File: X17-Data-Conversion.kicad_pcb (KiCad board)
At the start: 2 copper layers, 41.5 x 30.7 mm, 28 parts, among them J1 Conn_01x05, J4 Conn_01x12_Pin, U2 STM32F091CCTx, U3 MAX485E, U4 MAX7375AXR805+T, U5 AZ1117IH-3.3TRG1

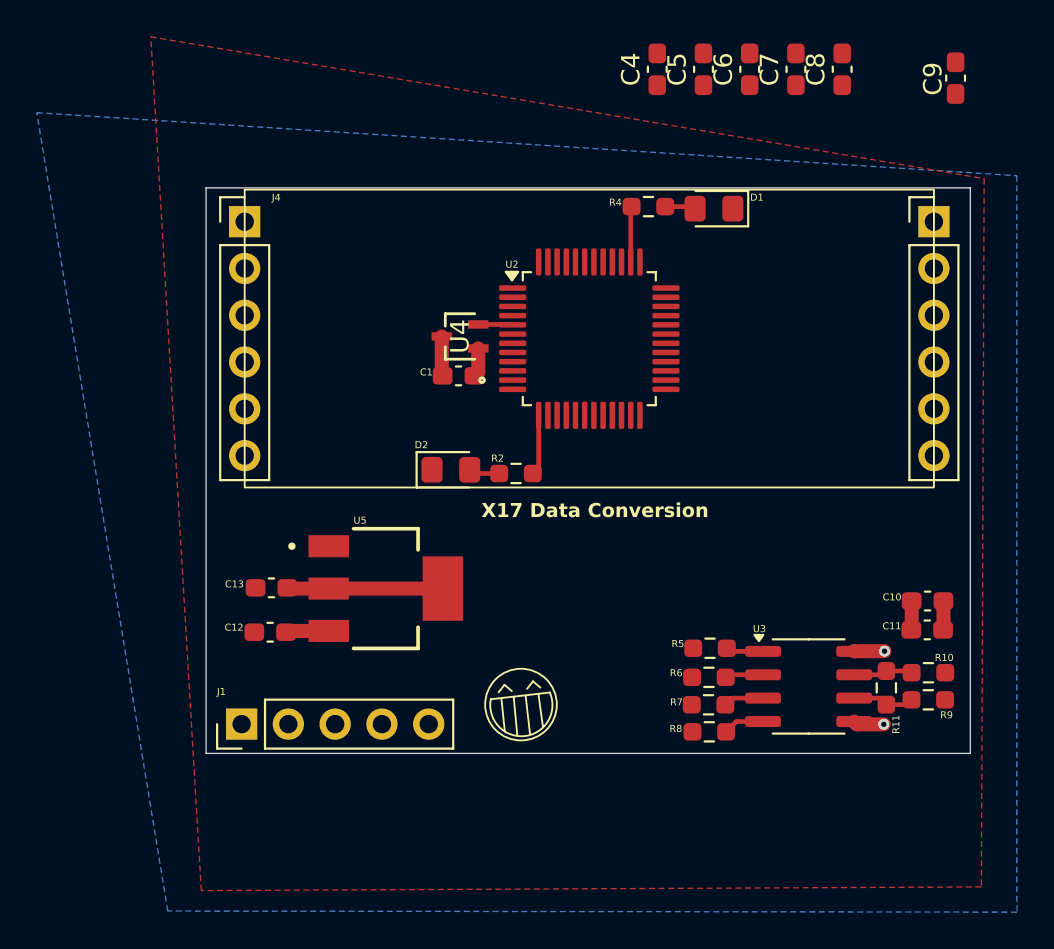
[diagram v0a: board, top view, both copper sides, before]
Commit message: goodie
going good
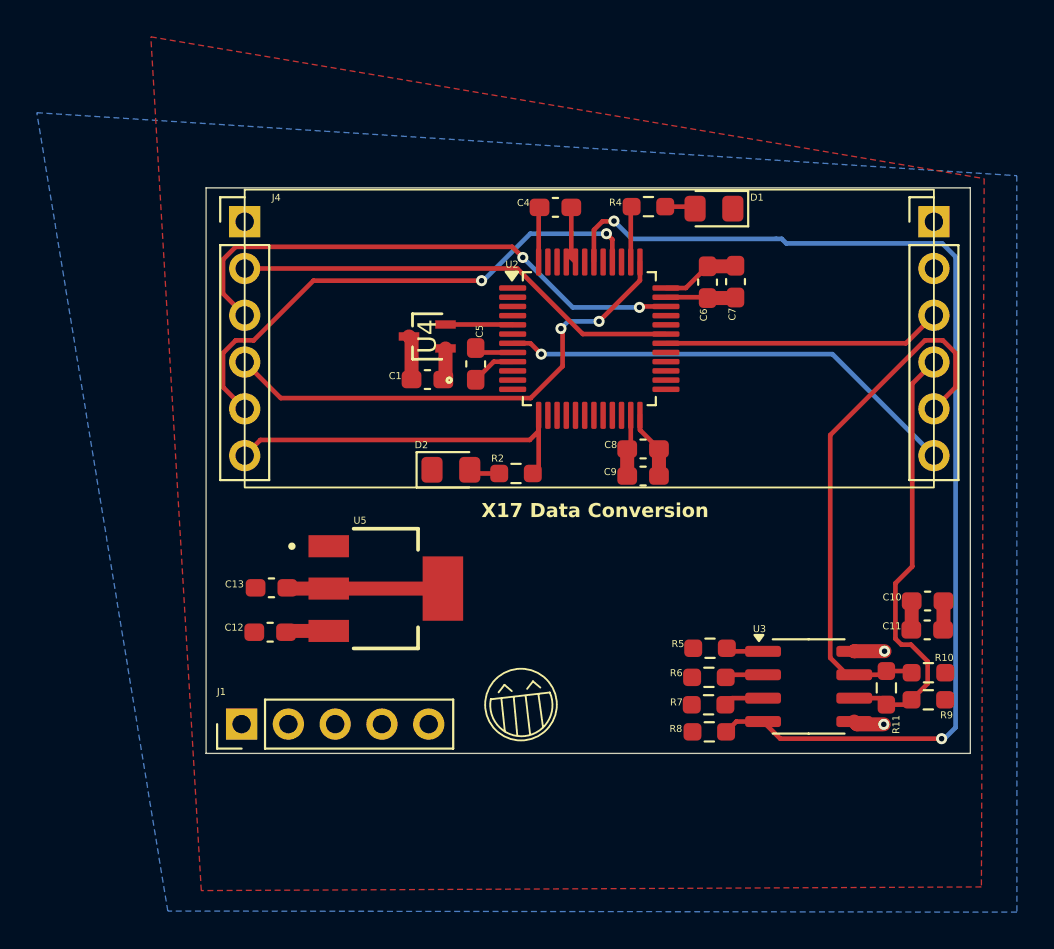
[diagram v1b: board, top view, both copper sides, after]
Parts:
- moved C9 27.5 mm to (164.5, 81.7), turned to 0 degrees
- moved C8 23.3 mm to (164.5, 80.2), turned to 0 degrees
- moved C5 20.2 mm to (155.4, 75.6), turned to -90 degrees
- moved C7 12.0 mm to (169.5, 71.1)
- moved C6 11.8 mm to (168.0, 71.1)
- moved C4 9.32 mm to (159.7, 67.1), turned to 180 degrees
- moved U4 1.78 mm to (152.8, 74.1)
- moved C1 1.70 mm to (152.8, 76.4)
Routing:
- net USART1_TX: track 2.24 -> 61.6 mm, vias 0 -> 2
- net SWDIO: track 0.00 -> 29.4 mm, vias 0 -> 2
- net ALERT1: track 0.00 -> 28.7 mm, vias 0 -> 2
- net SWCLK: track 0.00 -> 27.4 mm, vias 0 -> 2
- net A-: track 3.24 -> 29.8 mm
- net NRST_PSB: track 0.00 -> 25.4 mm, vias 0 -> 1
- net I2C1_SDA: track 0.00 -> 24.3 mm
- net A+: track 3.36 -> 24.0 mm
- net PG: track 3.29 -> 20.7 mm
- net I2C1_SCL: track 0.00 -> 15.2 mm
- net 3.3V: track 10.0 -> 23.6 mm
- net GND: track 5.40 -> 18.0 mm
- net Net-(U2-PF0): track 1.88 -> 3.66 mm
